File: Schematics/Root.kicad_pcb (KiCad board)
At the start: 2 copper layers, 100 x 100 mm, 139 parts, among them CON1 USB-MICRO-B, CON2 BARREL_JACK, IC1 ATXMEGA256A3BU-A, J1 AVR_JTAG_Header, P1 CONN_02X08, SW1 SW_PUSH, SW2 SW_PUSH, SW3 SW_PUSH, SW4 SW_PUSH, U1 PCA9685, U10 PCA9685, U11 PCA9685, U12 PCA9685, U13 LT8612, U2 PCA9685, U3 PCA9685, U4 PCA9685, U5 PCA9685, U6 PCA9685, U7 PCA9685, U8 PCA9685, U9 PCA9685, X1 16MHz, X2 32.768KhZ

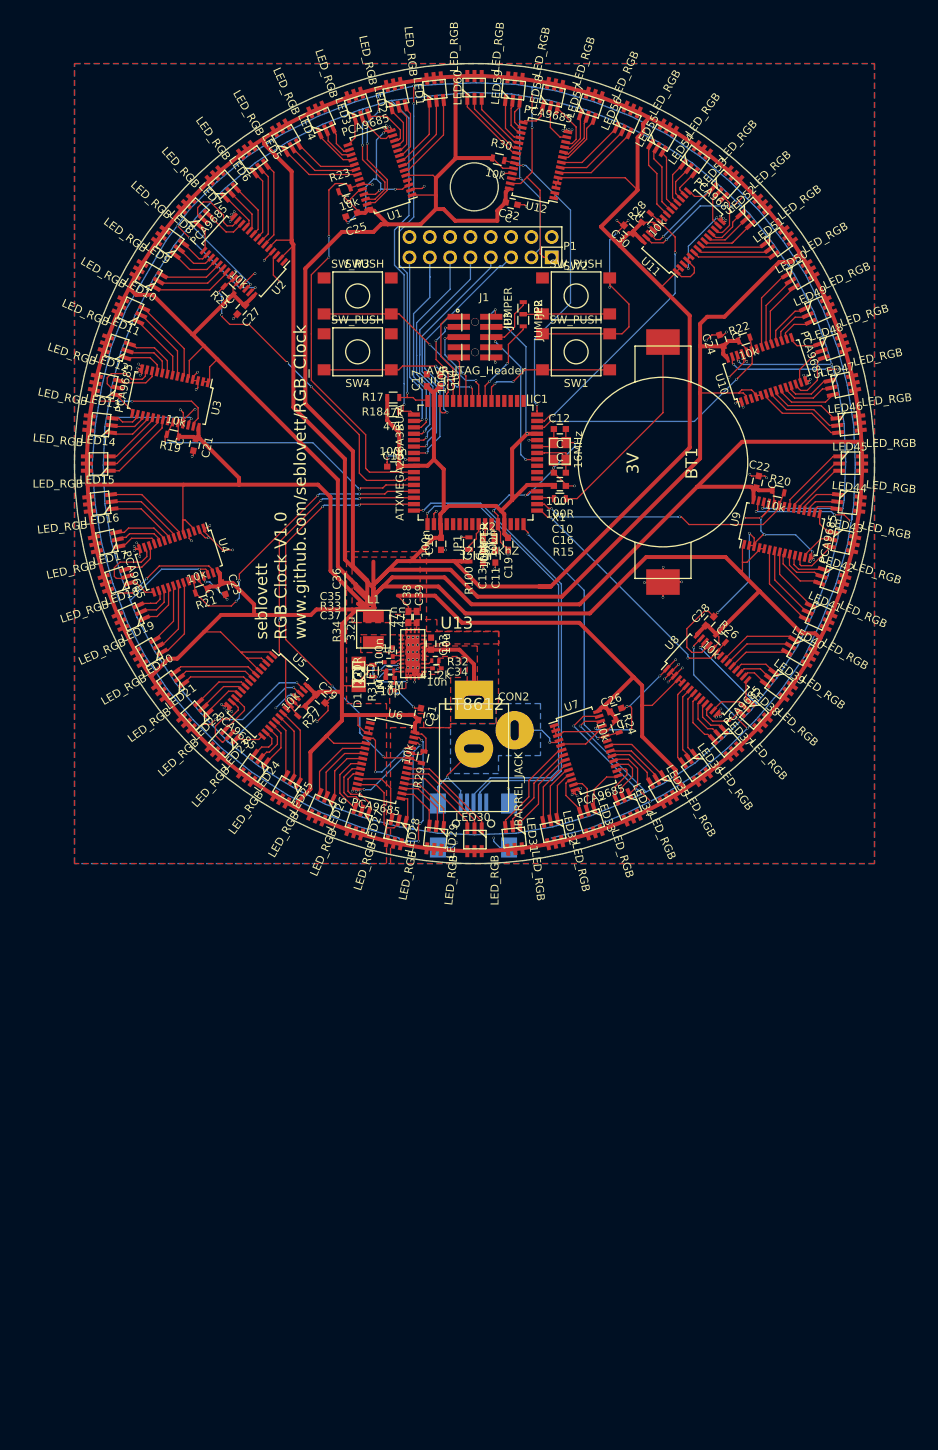
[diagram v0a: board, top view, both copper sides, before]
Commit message: Started Redesign.
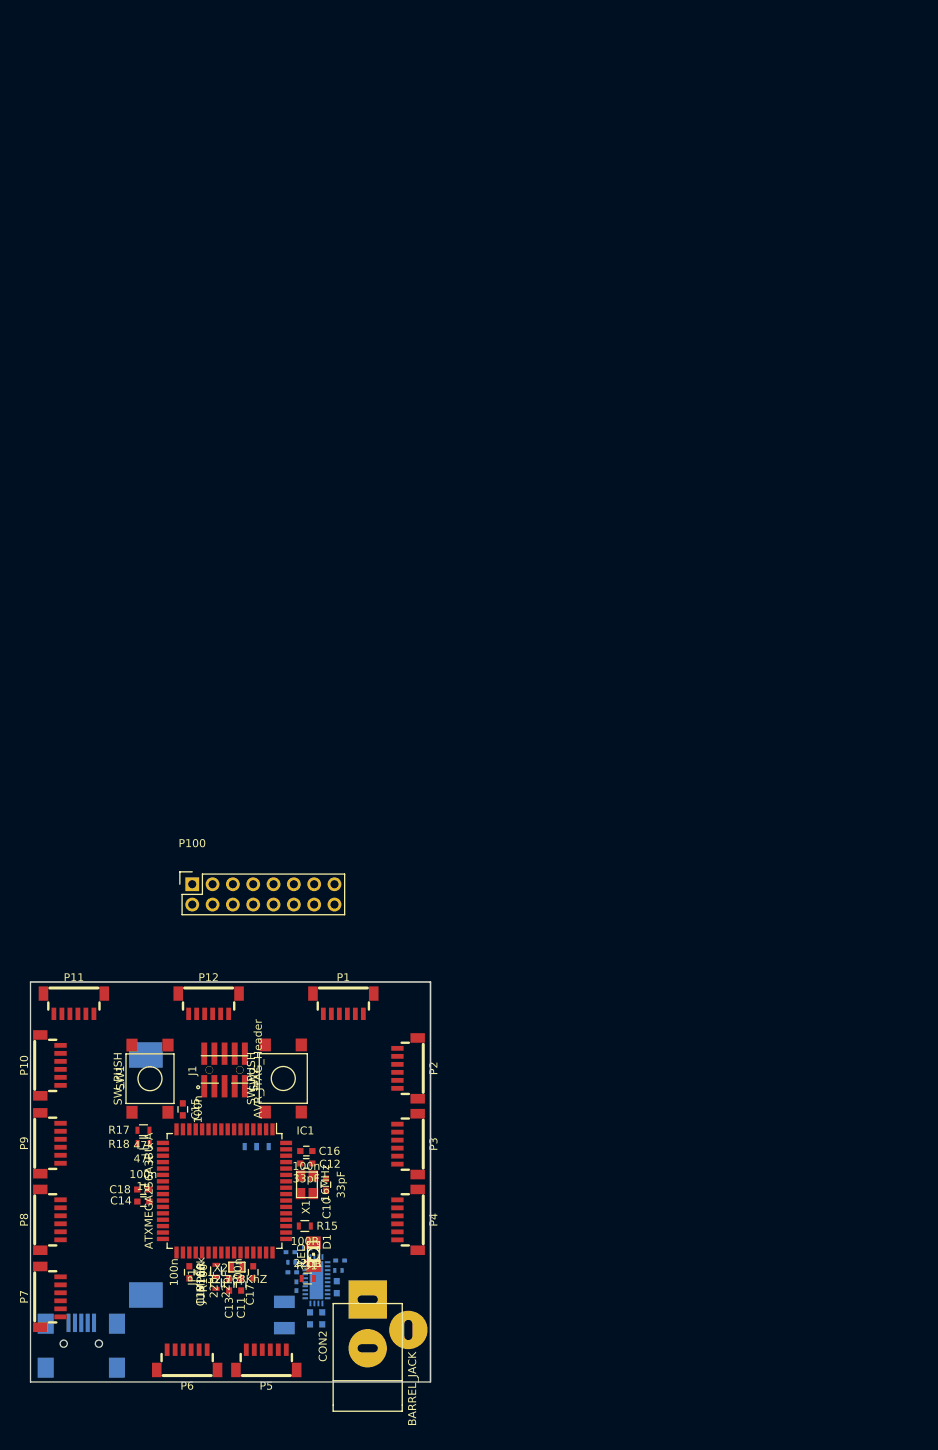
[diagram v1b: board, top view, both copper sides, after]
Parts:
- removed C21, C22, C23, C24, C25, C26, C27, C28, C29, C30, C31, C32: C, Capacitors_SMD:C_0603
- removed LED1, LED10, LED11, LED12, LED13, LED14, LED15, LED16, LED17, LED18, LED19, LED2, LED20, LED21, LED22, LED23, LED24, LED25, LED26, LED27, LED28, LED29, LED3, LED30, LED31, LED32, LED33, LED34, LED35, LED36, LED37, LED38, LED39, LED4, LED40, LED41, LED42, LED43, LED44, LED45, LED46, LED47, LED48, LED49, LED5, LED50, LED51, LED52, LED53, LED54, LED55, LED56, LED57, LED58, LED59, LED6, LED60, LED7, LED8, LED9: LED_RGB, rgb:rgbled1
- removed R19, R20, R21, R22, R23, R24, R25, R26, R27, R28, R29, R30: 10k, Resistors_SMD:R_0603
- removed SW3, SW4: SW_PUSH, rgb:SW
- removed U1, U10, U11, U12, U2, U3, U4, U5, U6, U7, U8, U9: PCA9685, Housings_SSOP:TSSOP-28_4.4x9.7mm_Pitch0.65mm
- added P10: CONN_01X06, JST-SH:JST-BM-06B-SRSS-TB, F.Cu at (52.2, 160.4)
- added P100: CONN_02X08, Socket_Strips:Socket_Strip_Straight_2x08, F.Cu at (70.2, 137.8)
- added P11: CONN_01X06, JST-SH:JST-BM-06B-SRSS-TB, F.Cu at (55.4, 152.5)
- added P12: CONN_01X06, JST-SH:JST-BM-06B-SRSS-TB, F.Cu at (72.3, 152.5)
- added P2: CONN_01X06, JST-SH:JST-BM-06B-SRSS-TB, F.Cu at (97.4, 160.8)
- added P3: CONN_01X06, JST-SH:JST-BM-06B-SRSS-TB, F.Cu at (97.4, 170.3)
- added P4: CONN_01X06, JST-SH:JST-BM-06B-SRSS-TB, F.Cu at (97.4, 179.7)
- added P5: CONN_01X06, JST-SH:JST-BM-06B-SRSS-TB, F.Cu at (79.5, 197.5)
- added P6: CONN_01X06, JST-SH:JST-BM-06B-SRSS-TB, F.Cu at (69.6, 197.5)
- added P7: CONN_01X06, JST-SH:JST-BM-06B-SRSS-TB, F.Cu at (52.2, 189.4)
- added P8: CONN_01X06, JST-SH:JST-BM-06B-SRSS-TB, F.Cu at (52.2, 179.7)
- added P9: CONN_01X06, JST-SH:JST-BM-06B-SRSS-TB, F.Cu at (52.2, 170.2)
- BT1, C33, C34, C35, C36, C37, C38, C39, JP2, JP3, L1, R32, R33, R34, U13: moved to B.Cu
- C10, C12: value C -> 33pF
- C11, C13: value C -> 22pF
- P1: value CONN_02X08 -> CONN_01X06; footprint Socket_Strips:Socket_Strip_Straight_2x08 -> JST-SH:JST-BM-06B-SRSS-TB
- moved C17 113.6 mm to (77.8, 186.3), turned to 270 degrees
- moved BT1 110.1 mm to (64.4, 174.1)
- moved JP2 109.8 mm to (79.0, 170.6), turned to 180 degrees
- moved C14 109.1 mm to (64.1, 177.4), turned to 180 degrees
- moved JP3 108.8 mm to (77.5, 170.6), turned to 0 degrees
- moved SW1 105.3 mm to (64.9, 162.1), turned to 270 degrees
- moved SW2 104.4 mm to (81.6, 162.1), turned to 270 degrees
- moved C19 99.4 mm to (69.8, 186.3)
- moved JP1 97.7 mm to (73.2, 187.6), turned to 270 degrees
- moved C12 97.1 mm to (84.5, 172.7)
- moved X1 97.0 mm to (84.6, 175.3)
- moved J1 96.8 mm to (74.3, 161.0), turned to 90 degrees
- moved R17 96.8 mm to (64.1, 168.5)
- moved R18 96.7 mm to (64.1, 170.2)
- moved C11 96.4 mm to (76.3, 187.8)
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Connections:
- net /Display/SCL renamed /Microcontroller/SCL
- CON1 pad 1: Net-(CON1-Pad1) -> (no net)
- IC1 pad 1: Net-(IC1-Pad1) -> (no net)
- IC1 pad 16: /Display/SDA -> /Microcontroller/SDA
- IC1 pad 2: Net-(IC1-Pad2) -> (no net)
- IC1 pad 26: /Display/Display Sub block 1/~OE -> (no net)
- IC1 pad 27: /Display/Display Sub block 2/~OE -> (no net)
- IC1 pad 28: /Display/Display Sub block 3/~OE -> (no net)
- IC1 pad 29: /Display/Display Sub block 4/~OE -> (no net)
- IC1 pad 3: Net-(IC1-Pad3) -> (no net)
- IC1 pad 30: /Display/Display Sub block 5/~OE -> (no net)
- IC1 pad 31: /Display/Display Sub block 6/~OE -> (no net)
- IC1 pad 36: Net-(IC1-Pad36) -> (no net)
- IC1 pad 37: Net-(IC1-Pad37) -> (no net)
- IC1 pad 38: Net-(IC1-Pad38) -> (no net)
- IC1 pad 39: Net-(IC1-Pad39) -> (no net)
- IC1 pad 4: Net-(IC1-Pad4) -> (no net)
- IC1 pad 40: Net-(IC1-Pad40) -> (no net)
- IC1 pad 46: Net-(IC1-Pad46) -> (no net)
- IC1 pad 47: Net-(IC1-Pad47) -> (no net)
- IC1 pad 48: /Display/Display Sub block 7/~OE -> (no net)
- IC1 pad 49: /Display/Display Sub block 8/~OE -> (no net)
- IC1 pad 5: Net-(IC1-Pad5) -> (no net)
- IC1 pad 50: /Display/Display Sub block 9/~OE -> (no net)
- IC1 pad 54: Net-(IC1-Pad54) -> (no net)
- IC1 pad 55: Net-(IC1-Pad55) -> (no net)
- IC1 pad 56: Net-(IC1-Pad56) -> (no net)
- IC1 pad 62: /Display/Display Sub block 10/~OE -> (no net)
- IC1 pad 63: /Display/Display Sub block 11/~OE -> (no net)
- IC1 pad 64: /Display/Display Sub block 12/~OE -> (no net)
- J1 pad 7: Net-(J1-Pad7) -> (no net)
- J1 pad 8: Net-(J1-Pad8) -> (no net)
- P1 pad 1: /Display/SDA -> VPP
- P1 pad 2: GND -> /Microcontroller/SDA
- P1 pad 5: /Microcontroller/SCK -> (no net)
- R17 pad 2: /Display/SDA -> /Microcontroller/SDA
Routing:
- net VPP: track 1373.7 -> 0.00 mm, vias 4 -> 0
- net /Display/SDA: track 518.5 -> 0.00 mm, vias 39 -> 0
- net /Microcontroller/SCL: track 492.5 -> 0.00 mm, vias 14 -> 0
- net GND: track 391.0 -> 0.00 mm, vias 150 -> 0
- net /Microcontroller/USB_D-: track 59.0 -> 0.00 mm, vias 1 -> 0
- net /Microcontroller/USB_D+: track 58.2 -> 0.00 mm, vias 1 -> 0
- net /Display/Display Sub block 6/~OE: track 54.9 -> 0.00 mm, vias 6 -> 0
- net /Display/Display Sub block 1/~OE: track 51.2 -> 0.00 mm, vias 3 -> 0
- net /Display/Display Sub block 5/~OE: track 42.5 -> 0.00 mm, vias 4 -> 0
- net /Display/Display Sub block 2/~OE: track 41.3 -> 0.00 mm, vias 7 -> 0
- net /Display/Display Sub block 12/~OE: track 38.3 -> 0.00 mm, vias 2 -> 0
- net /Display/Display Sub block 4/~OE: track 37.6 -> 0.00 mm, vias 4 -> 0
- net /Display/Display Sub block 3/~OE: track 36.6 -> 0.00 mm, vias 2 -> 0
- net /Display/Display Sub block 11/~OE: track 35.2 -> 0.00 mm, vias 2 -> 0
- net /Display/Display Sub block 9/~OE: track 34.2 -> 0.00 mm, vias 2 -> 0
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- removed copper zone on F.Cu, net /Power Supply/SW
- removed copper zone on F.Cu, net /Power Supply/Vin
- removed copper zone on B.Cu, net GND
- removed copper zone on F.Cu, net GND
- removed copper zone on F.Cu, net VPP
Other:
- board size 100 x 100 mm -> 50 x 50 mm
- net class Default: clearance 0.15 -> 0.254; trace_width 0.15 -> 0.254; via_dia 0.3 -> 0.889; via_drill 0.25 -> 0.635
- net class Power removed
- rule trace_clearance: 0.15 -> 0.254
- rule trace_min: 0.15 -> 0.254
- rule via_min_drill: 0.25 -> 0.508
- rule via_min_size: 0.3 -> 0.889
- board text removed: "Absolute maximum current all LEDs can draw is 6A. Averages to 0.55A per track. At this rating, need at least 0.12mm track for 10C rise. We have 0.5 so easily safe"
- board text removed: "Vin track - 3A 10C rise 4A 20C rise. 6A - 50C rise. Getting too hot for this, but cannot afford a thicker track."
- board text removed: "seblovett RGB Clock V1.0 www.github.com/seblovett/RGB_Clock"
